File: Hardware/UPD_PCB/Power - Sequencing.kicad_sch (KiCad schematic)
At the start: 0 parts

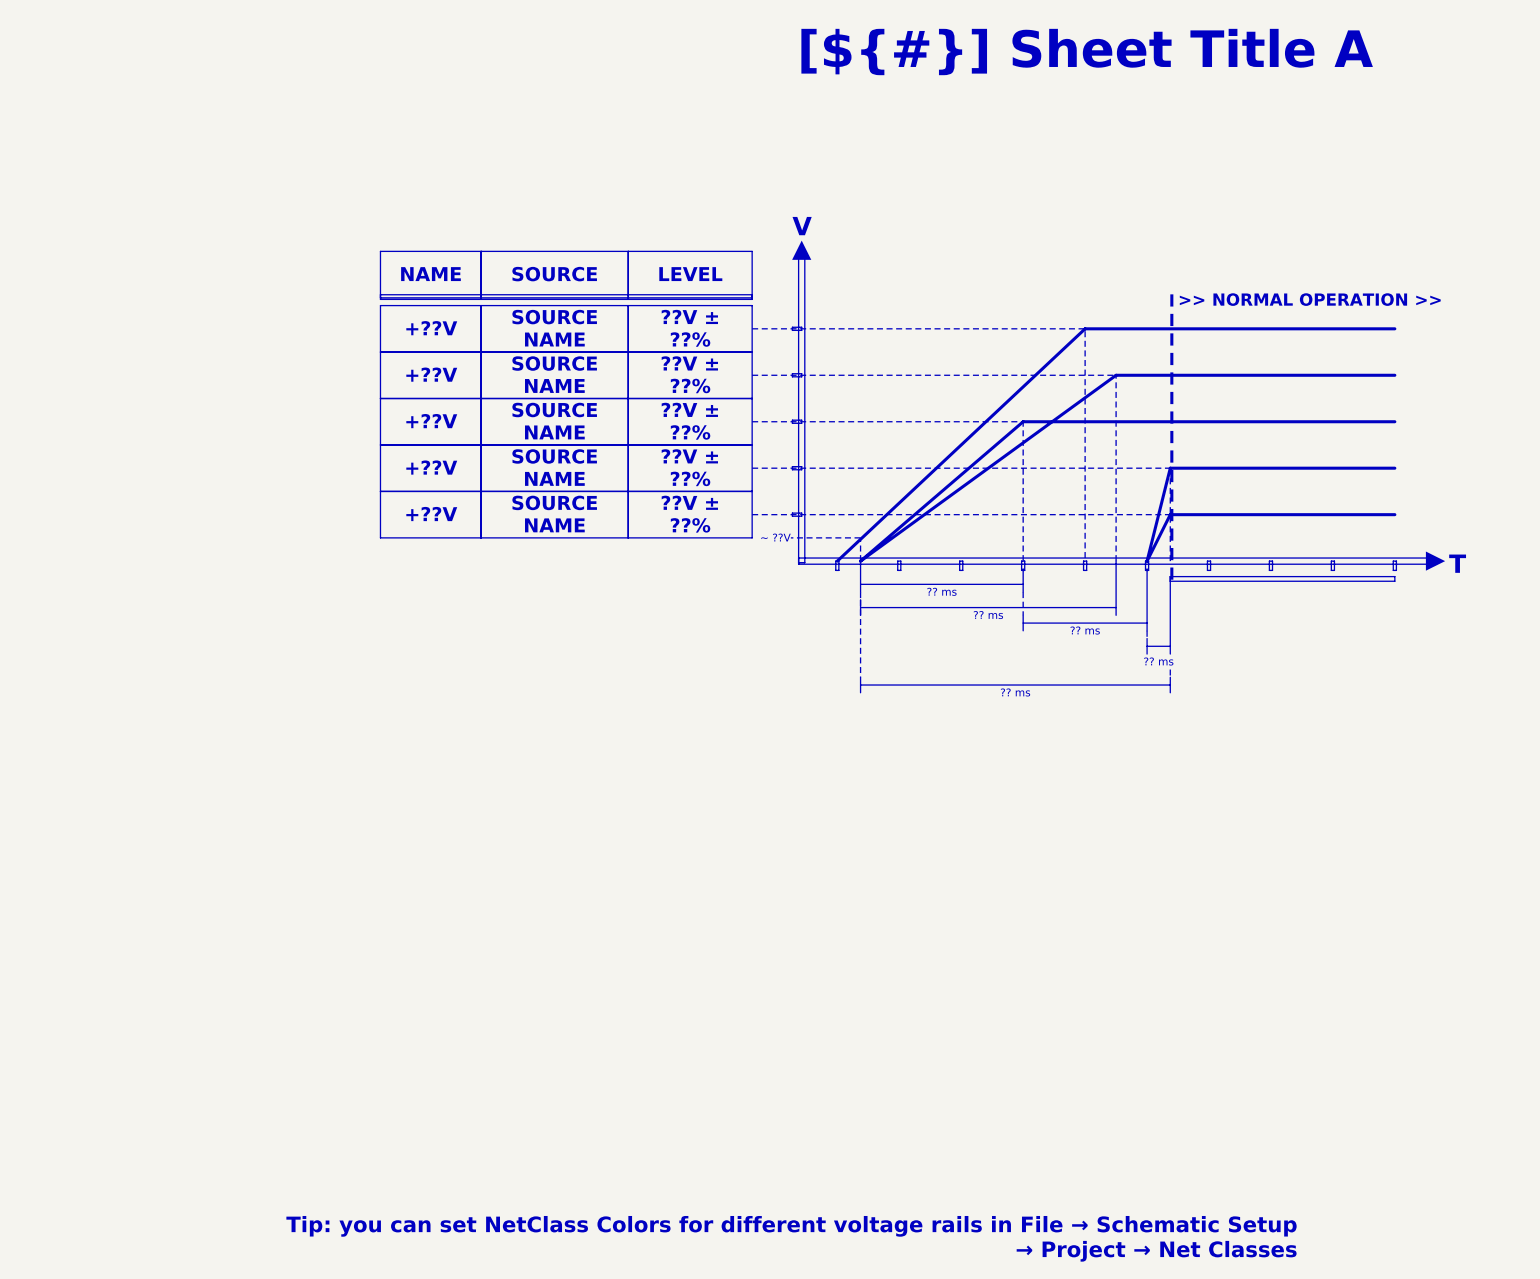
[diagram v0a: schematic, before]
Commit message: Finalized version V1.0
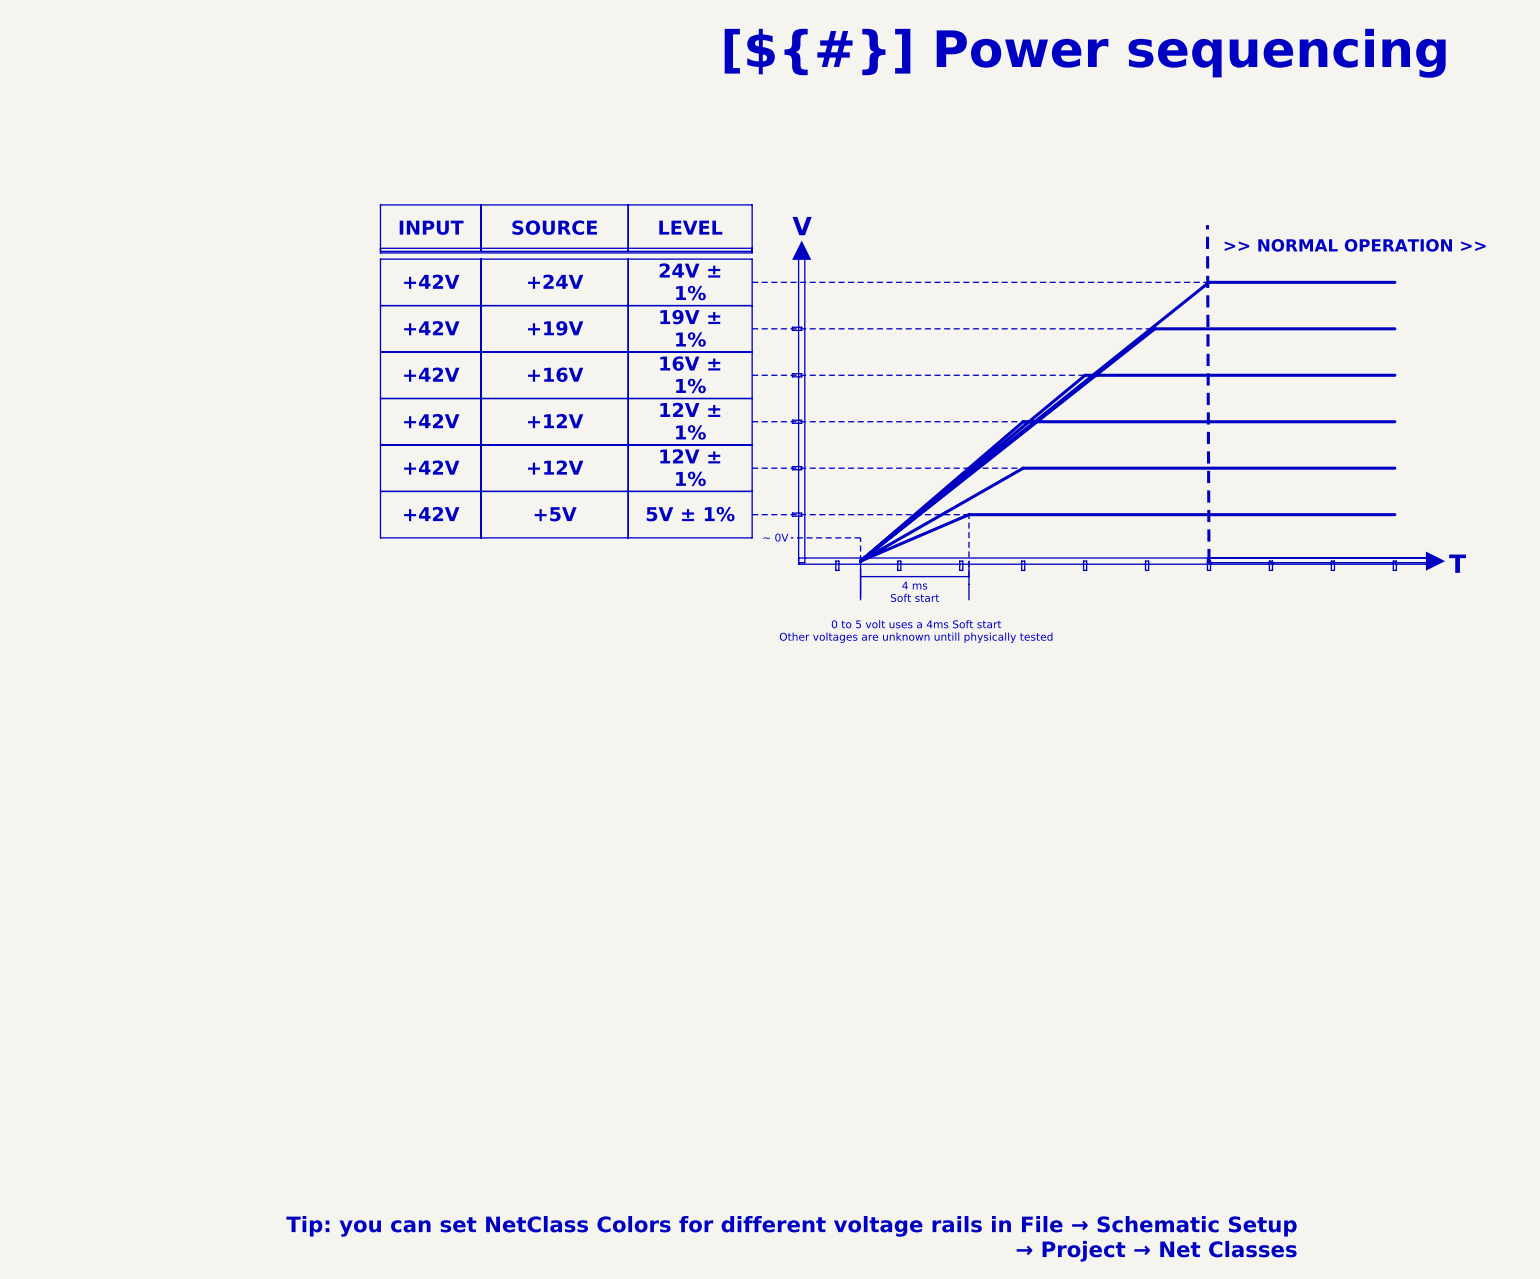
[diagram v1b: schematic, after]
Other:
- note added: "0 to 5 volt uses a 4ms Soft start Other voltages are unknown untill physically tested"
